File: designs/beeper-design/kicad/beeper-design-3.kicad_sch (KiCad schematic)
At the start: 30 parts, among them U12 DRV2605YZFR, U13 CSD75207W15, U3 BQ51003YFPR

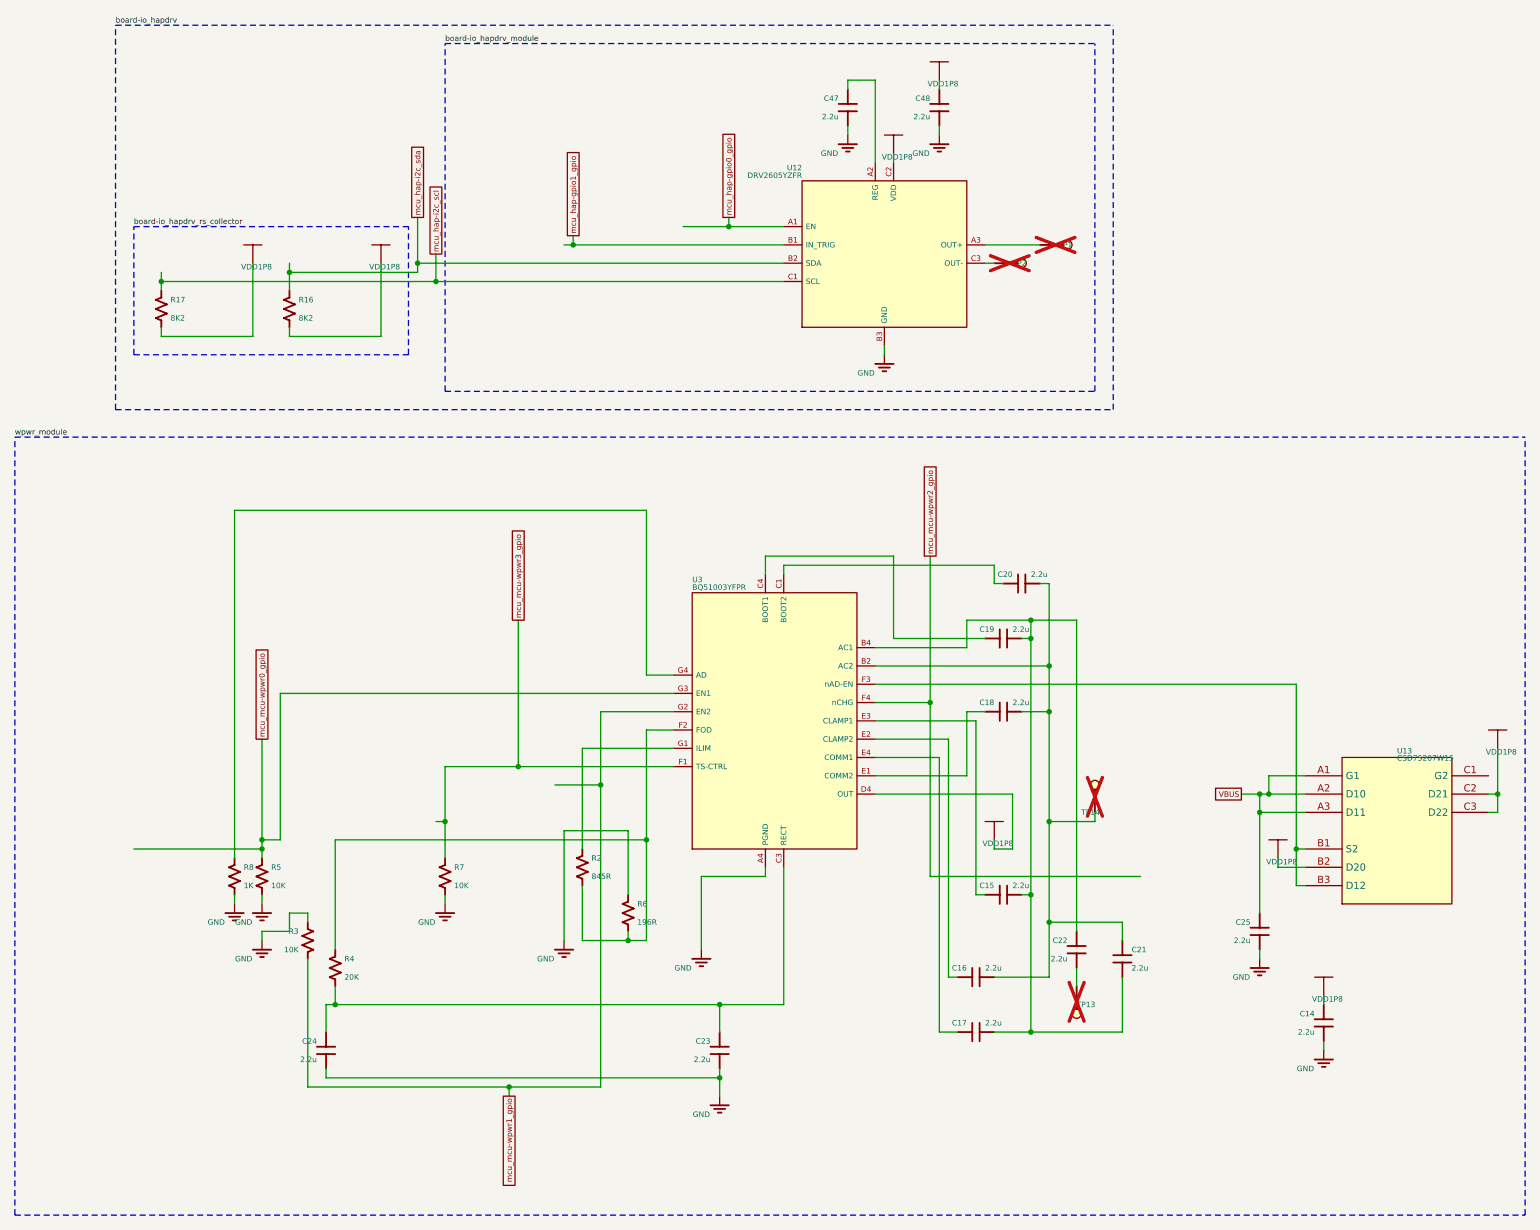
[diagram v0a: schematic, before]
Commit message: another export
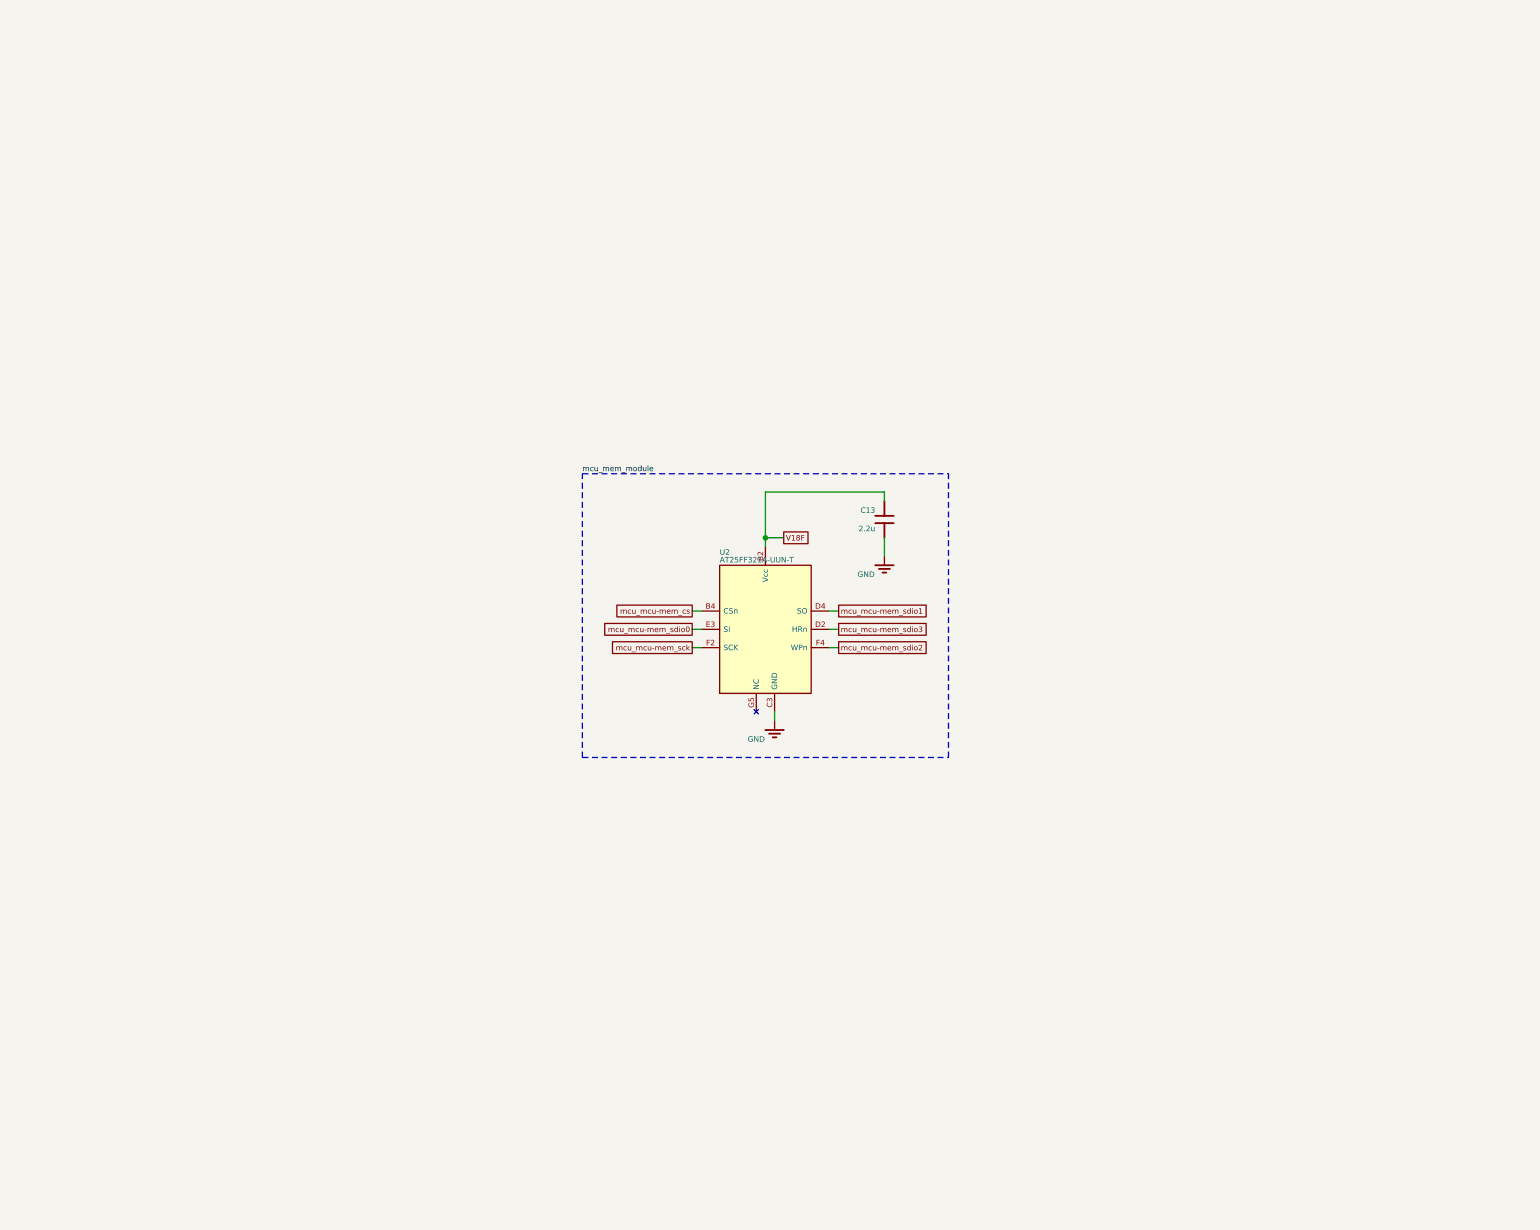
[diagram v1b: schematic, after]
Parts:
- removed C14: 2.2u, beeper-design:Pkg0201_18, symbol C335106_9
- removed C15: 2.2u, beeper-design:Pkg0201_11, symbol C335106_5
- removed C16: 2.2u, beeper-design:Pkg0201_27, symbol C335106_17
- removed C17: 2.2u, beeper-design:Pkg0201_40, symbol C335106_26
- removed C18: 2.2u, beeper-design:Pkg0201_53, symbol C335106_35
- removed C19: 2.2u, beeper-design:Pkg0201_10, symbol C335106_4
- removed C20: 2.2u, beeper-design:Pkg0201_26, symbol C335106_16
- removed C21: 2.2u, beeper-design:Pkg0201_39, symbol C335106_25
- removed C22: 2.2u, beeper-design:Pkg0201_52, symbol C335106_34
- removed C23: 2.2u, beeper-design:Pkg0201_9, symbol C335106_3
- removed C24: 2.2u, beeper-design:Pkg0201_23, symbol C335106_13
- removed C25: 2.2u, beeper-design:Pkg0201_16, symbol C335106_7
- removed C47: 2.2u, beeper-design:Pkg0201_35, symbol C335106_23
- removed C48: 2.2u, beeper-design:Pkg0201_47, symbol C335106_29
- removed R16, R17: 8K2, beeper-design:Pkg0201_8, symbol my_resistor_3
- removed R2: 845R, beeper-design:Pkg0201_32, symbol my_resistor_7
- removed R3: 10K, beeper-design:Pkg0201_30, symbol my_resistor_6
- removed R4: 20K, beeper-design:Pkg0201_2, symbol my_resistor
- removed R5: 10K, beeper-design:Pkg0201_15, symbol my_resistor_4
- removed R6: 196R, beeper-design:Pkg0201_45, symbol C138167
- removed R7: 10K, beeper-design:Pkg0201_41, symbol my_resistor_9
- removed R8: 1K, beeper-design:Pkg0201_54, symbol my_resistor_12
- removed TP1, TP13, TP14, TP2: (no value), beeper-design:SMD_TESTPT, symbol smd_testpoint_cmp
- removed U12: DRV2605YZFR, beeper-design:LP_8, symbol DRV2605YZFR
- removed U13: CSD75207W15, beeper-design:LP_6, symbol CSD75207W15
- removed U3: BQ51003YFPR, beeper-design:LP_7, symbol BQ51003YFPR
- added C13: 2.2u, beeper-design:Pkg0201_34, symbol C335106_24
- added U2: AT25FF321A-UUN-T, beeper-design:WLCSP_12, symbol AT25FF321A_UUN_T
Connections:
- net GND: now also C13.1, U2.C3 (GND)
- new net: U2.A1 (NC), U2.A5 (NC), U2.G1 (NC), U2.G5 (NC)
- new net V18F: C13.2, U2.B2 (Vcc)
- new net mcu_mcu-mem_cs: U2.B4 (CSn)
- new net mcu_mcu-mem_sck: U2.F2 (SCK)
- new net mcu_mcu-mem_sdio0: U2.E3 (SI)
- new net mcu_mcu-mem_sdio1: U2.D4 (SO)
- new net mcu_mcu-mem_sdio2: U2.F4 (WPn)
- new net mcu_mcu-mem_sdio3: U2.D2 (HRn)
